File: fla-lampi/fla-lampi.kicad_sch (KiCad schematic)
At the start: 6 parts, among them J2 Conn_PinHeader_1x03_P2.54mm_H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, M2 Module_XIAO-RP2040, SW1 BUTTON_B3SN, SW2 BUTTON_B3SN

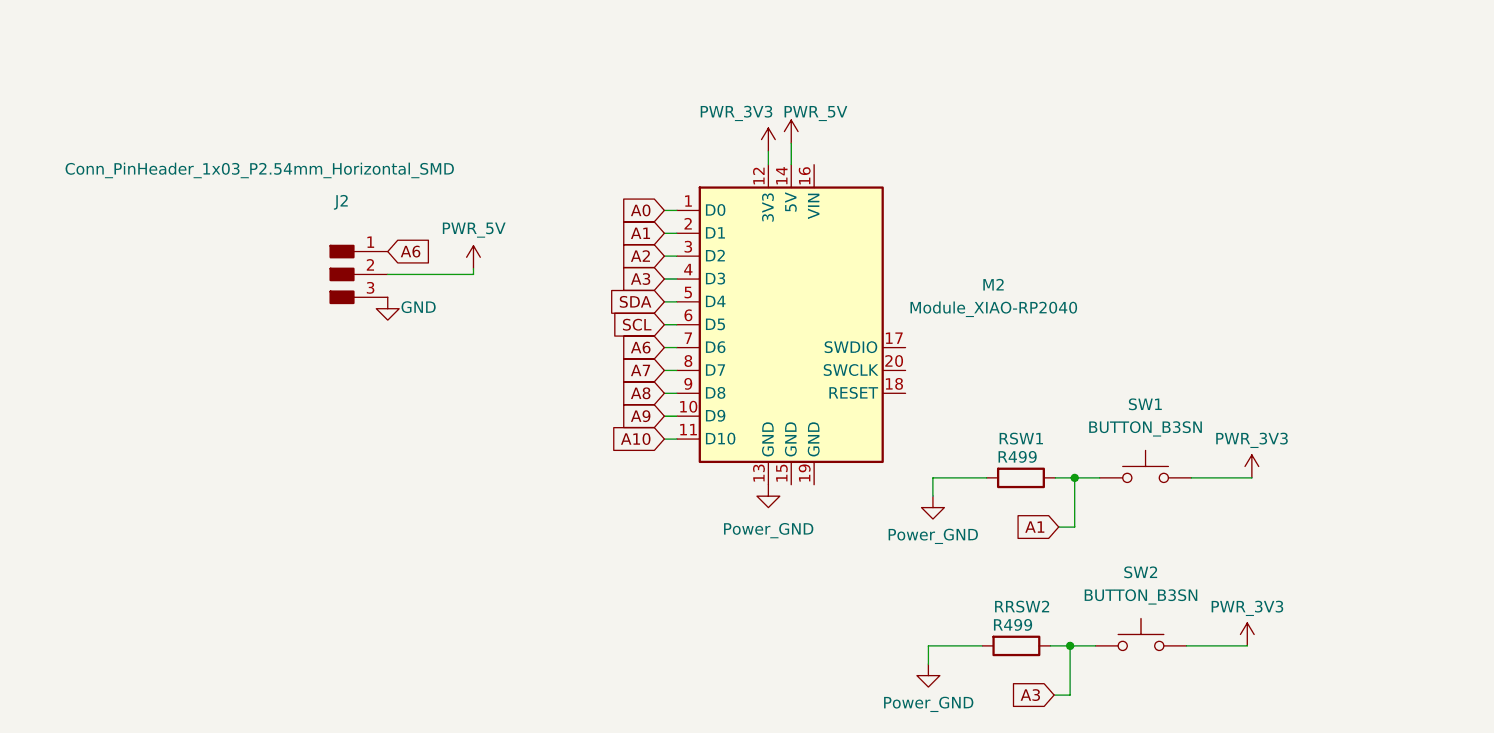
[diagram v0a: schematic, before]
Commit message: Myndir
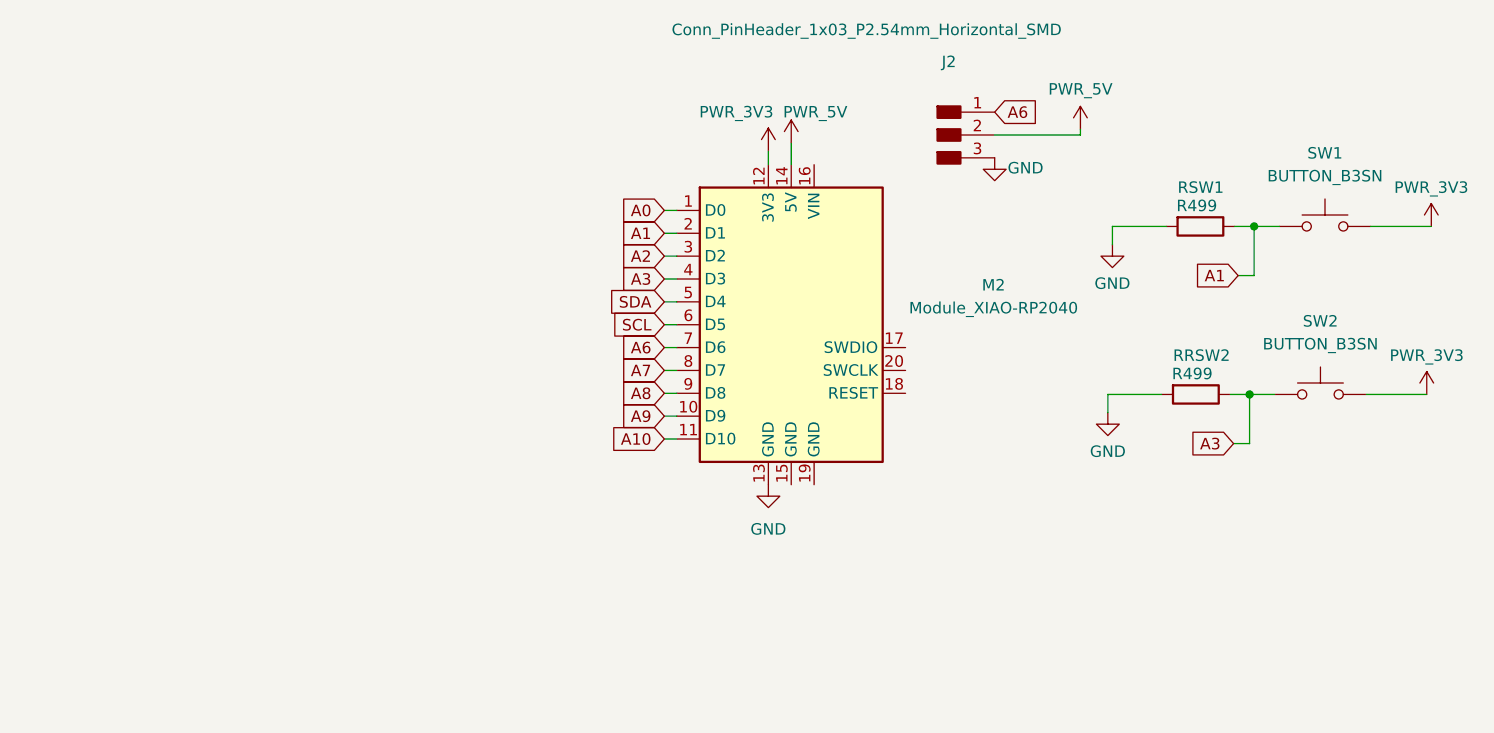
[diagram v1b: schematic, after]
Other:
- moved on the sheet: J2, RRSW2, RSW1, SW1, SW2
